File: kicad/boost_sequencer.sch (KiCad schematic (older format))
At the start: 54 parts, among them J1 Conn_01x05_Female, J2 Conn_01x03_Male, J3 Conn_01x07_Female, Q1 BC817, Q2 BC817, Q3 BC817, Q4 *P, Q5 *P, Q6 *N, Q7 *N, Q8 BC817, Q9 *P, U1 LM317_SOT-223, U2 ATtiny214-SS

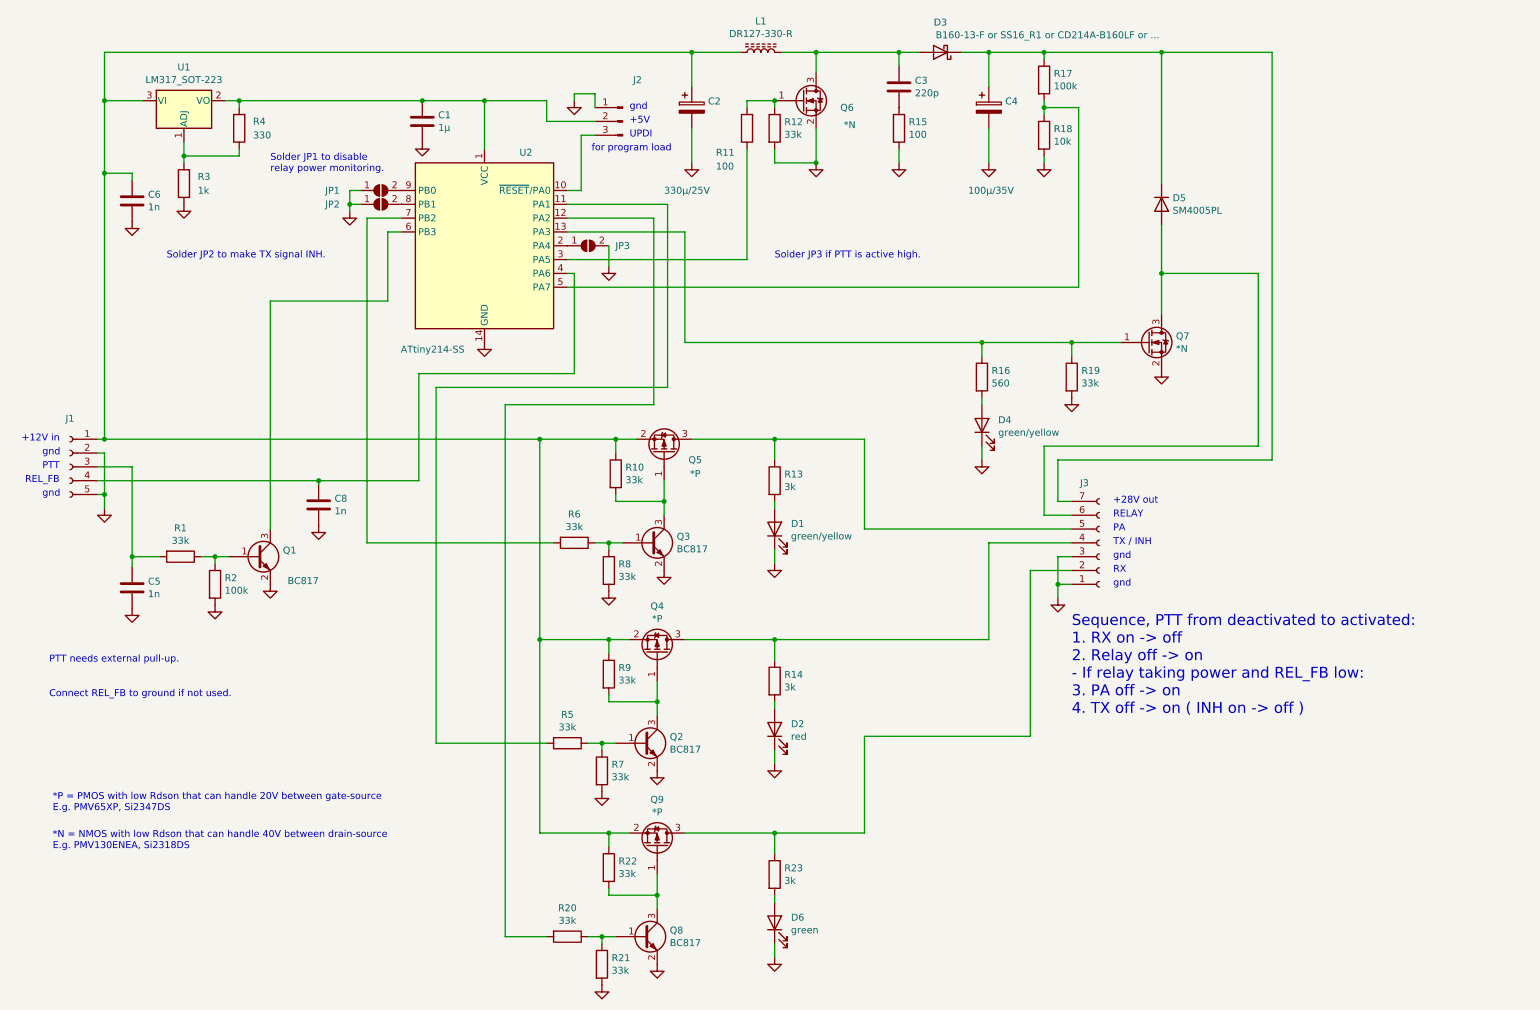
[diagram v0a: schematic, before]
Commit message: first on new board
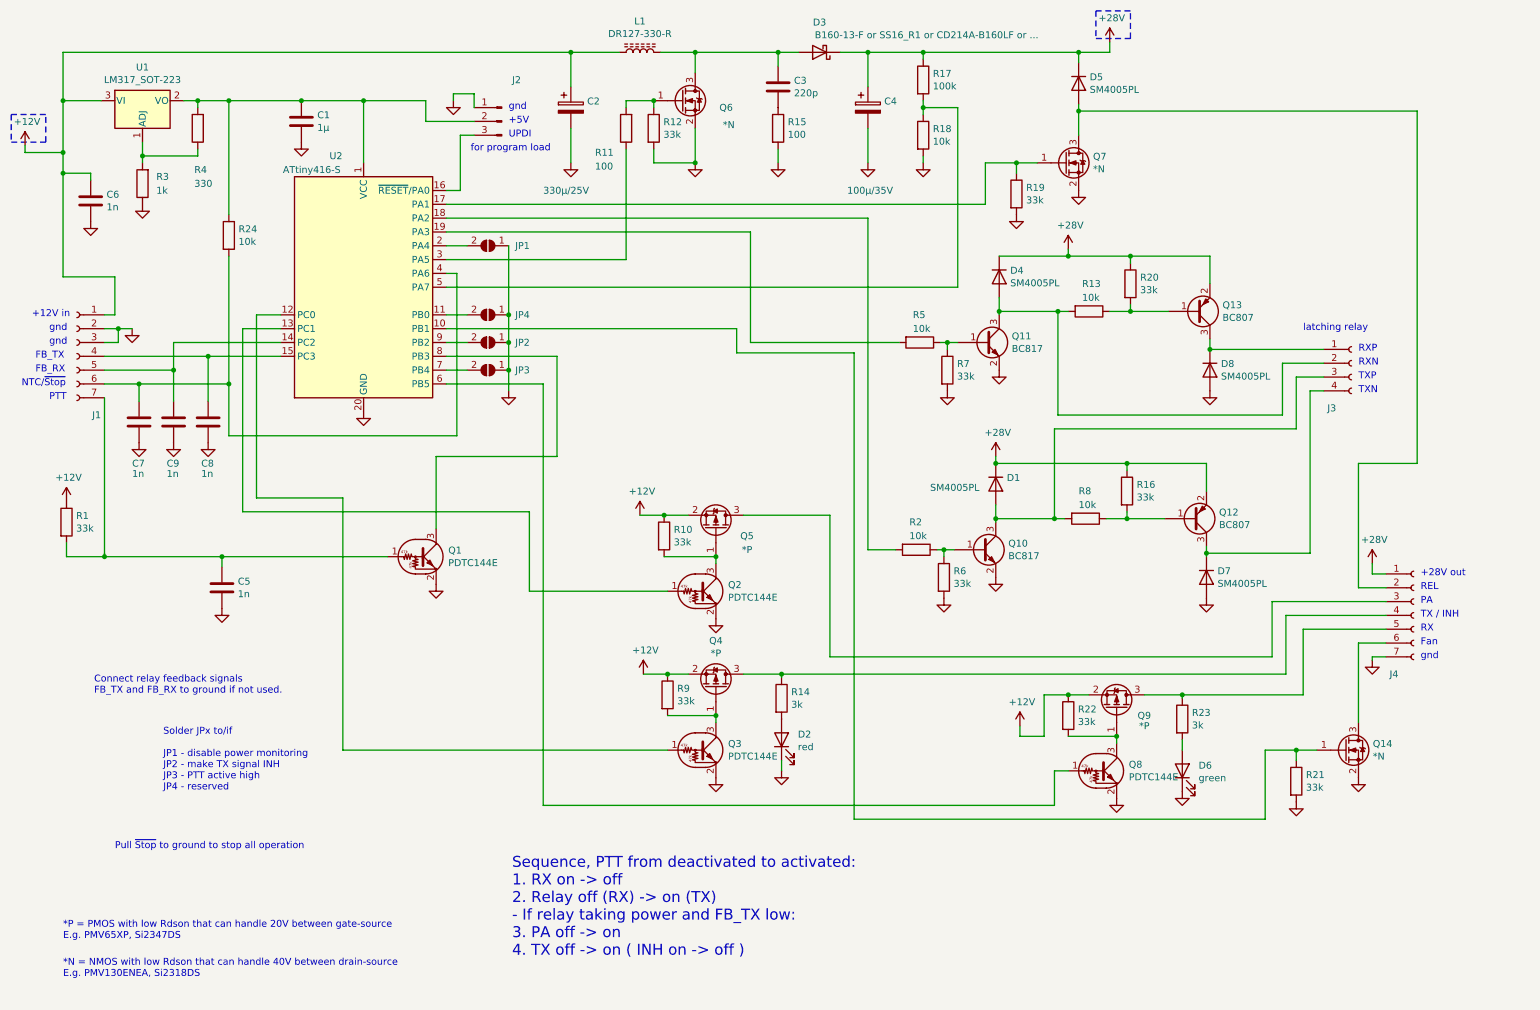
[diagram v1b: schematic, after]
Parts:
- removed D1, D4: green/yellow, LED_SMD:LED_0603_1608Metric, symbol Device:LED
- removed J1: Conn_01x05_Female, Connector_PinHeader_2.54mm:PinHeader_1x05_P2.54mm_Vertical, symbol Connector:Conn_01x05_Female
- removed J3: Conn_01x07_Female, Connector_PinHeader_2.54mm:PinHeader_1x07_P2.54mm_Vertical, symbol Connector:Conn_01x07_Female
- removed Q1, Q2, Q3, Q8: BC817, Package_TO_SOT_SMD:SOT-23, symbol Transistor_BJT:BC817
- removed U2: ATtiny214-SS, Package_SO:SOIC-14_3.9x8.7mm_P1.27mm, symbol MCU_Microchip_ATtiny:ATtiny414-SS
- added C7, C9: 1n, Capacitor_SMD:C_0603_1608Metric, symbol Device:C
- added D1, D4, D7, D8: SM4005PL, Diode_SMD:D_SOD-123F, symbol Device:D
- added J1, J4: Conn_01x07_Female, Connector_PinHeader_2.54mm:PinHeader_1x07_P2.54mm_Vertical, symbol Connector:Conn_01x07_Female
- added J3: Conn_01x04_Female, Connector_PinHeader_2.54mm:PinHeader_1x04_P2.54mm_Vertical, symbol Connector:Conn_01x04_Female
- added JP4: SolderJumper_2_Open, Jumper:SolderJumper-2_P1.3mm_Open_RoundedPad1.0x1.5mm, symbol Jumper:SolderJumper_2_Open
- added Q1, Q2, Q3, Q8: PDTC144E, Package_TO_SOT_SMD:SOT-323_SC-70, symbol Transistor_BJT:DTC144E
- added Q10, Q11: BC817, Package_TO_SOT_SMD:SOT-23, symbol Transistor_BJT:BC817
- added Q12, Q13: BC807, Package_TO_SOT_SMD:SOT-23, symbol Transistor_BJT:BC807
- added Q14: *N, Package_TO_SOT_SMD:SOT-23, symbol Device:Q_NMOS_GSD
- added R24: 10k, Resistor_SMD:R_0603_1608Metric, symbol Device:R
- added U2: ATtiny416-S, Package_SO:SOIC-20W_7.5x12.8mm_P1.27mm, symbol MCU_Microchip_ATtiny:ATtiny416-S
- R13: value 3k -> 10k
- R16: value 560 -> 33k
- R2: value 100k -> 10k
- R5, R8: value 33k -> 10k
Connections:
- net GND: now also JP3.1 (A), R6.2, C7.2, C9.2, D7.2 (A), D8.2 (A), J1.2 (Pin_2), J1.3 (Pin_3), J4.7 (Pin_7), JP4.1 (A), Q1.2 (E), Q10.2 (E), Q11.2 (E), Q14.2 (S), Q2.2 (E), Q3.2 (E), Q8.2 (E), U2.20 (GND); no longer JP3.2 (B), R2.2, R8.2
- net at C1.1, J2.2 (Pin_2), R4.2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: now also R24.1, U2.1 (VCC)
- net at J2.3 (Pin_3): now also U2.16 (~RESET~/PA0)
- net at R5.2: now also U2.19 (PA3)
- net at R20.2: now also R13.1, Q13.1 (B)
- net at Q7.1 (G), R19.1: now also U2.17 (PA1); no longer R16.1
- net at R11.1: now also U2.3 (PA5)
- net at C8.1: now also J1.4 (Pin_4), U2.15 (PC3)
- net at R17.2, R18.1: now also U2.5 (PA7)
- net at JP2.2 (B): now also U2.9 (PB2)
- net at JP1.2 (B): now also U2.2 (PA4)
- net +28V: now reaches C4.1, D3.1 (K), D5.1 (K), R17.1
- net +28V: now also R16.1, R20.1, D1.1 (K), D4.1 (K), J4.1 (Pin_1), Q12.2 (E), Q13.2 (E)
- net +12V: now reaches C2.1, C6.1, L1.1, Q4.2 (S), Q5.2 (S), Q9.2 (S), R10.1, R22.1, R9.1, U1.3 (VI)
- net +12V: now also R1.1, J1.1 (Pin_1)
- net at Q5.1 (G), R10.2: now also Q2.3 (C)
- net at Q5.3 (D): now also J4.3 (Pin_3); no longer R13.1
- net at R6.1: now also R2.1, Q10.1 (B); no longer R8.1
- net at Q4.1 (G), R9.2: now also Q3.3 (C)
- net at Q4.3 (D), R14.1: now also J4.4 (Pin_4)
- net at R5.1, R7.1: now also Q11.1 (B)
- net at D5.2 (A), Q7.3 (D): now also J4.2 (Pin_2)
- net at R13.2: now also D4.2 (A), J3.2 (Pin_2), Q11.3 (C)
- net at R16.2: now also R8.1, Q12.1 (B)
- net at C5.1, R1.2: now also J1.7 (Pin_7), Q1.1 (B)
- net at Q9.1 (G), R22.2: now also Q8.3 (C)
- net at Q9.3 (D), R23.1: now also J4.5 (Pin_5)
- net at R21.1: now also Q14.1 (G), U2.10 (PB1); no longer R20.1
- new net: JP3.2 (B), U2.7 (PB4)
- new net: JP4.2 (B), U2.11 (PB0)
- new net: Q3.1 (B), U2.12 (PC0)
- new net: Q2.1 (B), U2.13 (PC1)
- new net: C9.1, J1.5 (Pin_5), U2.14 (PC2)
- new net: R2.2, U2.18 (PA2)
- new net: C7.1, J1.6 (Pin_6), R24.2, U2.4 (PA6)
- new net: Q8.1 (B), U2.6 (PB5)
- new net: Q1.3 (C), U2.8 (PB3)
- new net: D8.1 (K), J3.1 (Pin_1), Q13.3 (C)
- new net: D7.1 (K), J3.4 (Pin_4), Q12.3 (C)
- new net: D1.2 (A), J3.3 (Pin_3), Q10.3 (C), R8.2
- new net: J4.6 (Pin_6), Q14.3 (D)
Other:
- note added: "Connect relay feedback signals\nFB_TX and FB_RX to ground if not used."
- note added: "FB_RX"
- note added: "FB_TX"
- note added: "Fan"
- note added: "NTC/~Stop"
- note added: "Pull ~Stop~ to ground to stop all operation"
- note added: "REL"
- note added: "RXN"
- note added: "RXP"
- note added: "Sequence, PTT from deactivated to activated:\n1. RX on -> off\n2. Relay off (RX) -> on (TX)\n- If relay taking power and FB_TX low:\n3. PA off -> on\n4. TX off -> on ( INH on -> off )"
- note added: "Solder JPx to/if\n\nJP1 - disable power monitoring\nJP2 - make TX signal INH\nJP3 - PTT active high\nJP4 - reserved\n"
- note added: "TXN"
- note added: "TXP"
- note added: "latching relay"
- note removed: "Connect REL_FB to ground if not used."
- note removed: "PTT needs external pull-up."
- note removed: "RELAY"
- note removed: "REL_FB"
- note removed: "Sequence, PTT from deactivated to activated:\n1. RX on -> off\n2. Relay off -> on\n- If relay taking power and REL_FB low:\n3. PA off -> on\n4. TX off -> on ( INH on -> off )"
- note removed: "Solder JP1 to disable\nrelay power monitoring."
- note removed: "Solder JP2 to make TX signal INH."
- note removed: "Solder JP3 if PTT is active high."
- moved on the sheet: C1, C2, C3, C4, C5, C6, C8, D2, D3, D5, D6, J2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
